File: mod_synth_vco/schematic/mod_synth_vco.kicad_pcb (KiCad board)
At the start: 2 copper layers, 38.1 x 109.2 mm, 29 parts, among them J1 Saw, J2 Triangle, J3 Conn_02x08_Odd_Even, J4 Freq CV, J5 PWM CV, J6 Square, U1 TL072, U2 AS3340, U3 TL072

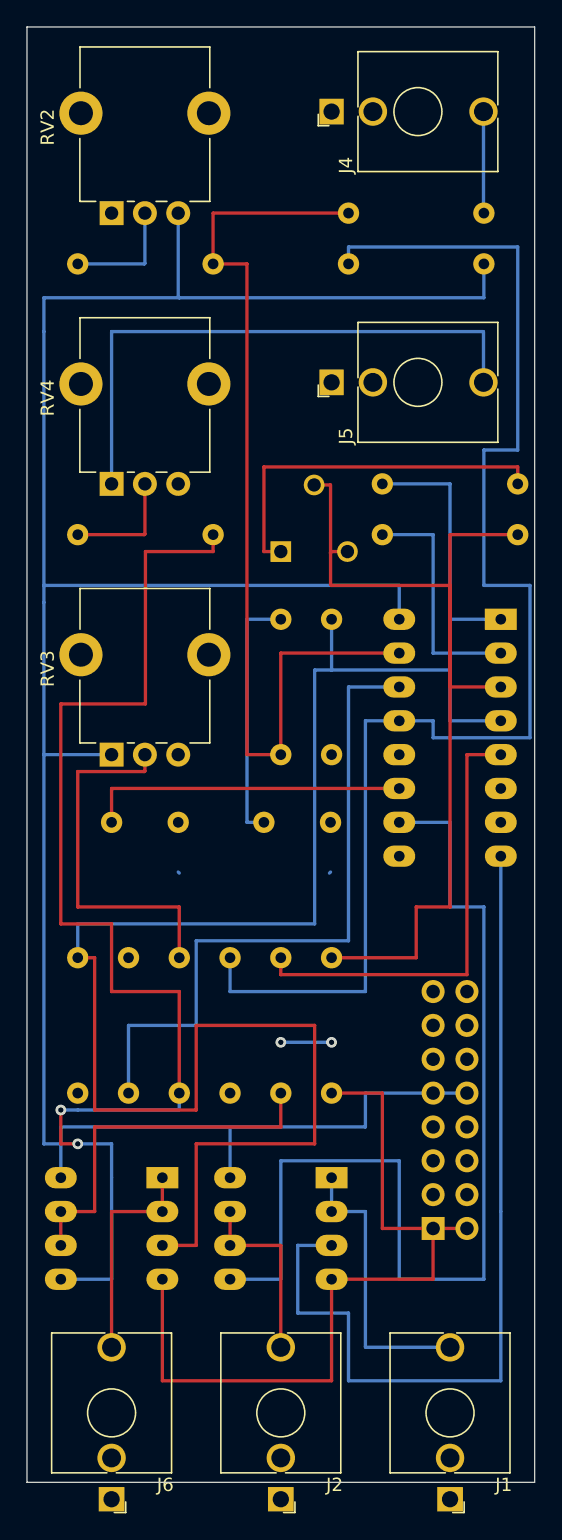
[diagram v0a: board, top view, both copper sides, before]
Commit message: Update PCB layouts
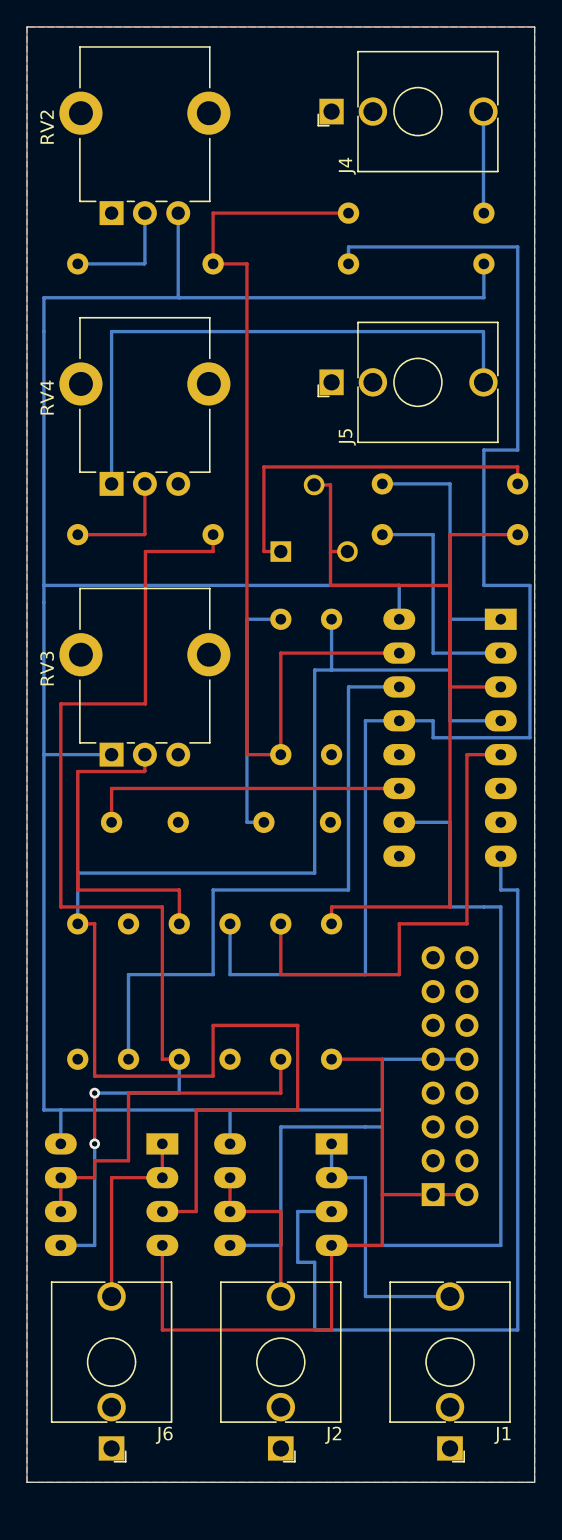
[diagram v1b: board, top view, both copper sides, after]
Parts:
- moved J1 3.81 mm to (69.8, 132.1)
- moved J2 3.81 mm to (57.1, 132.1)
- moved J6 3.81 mm to (44.5, 132.1)
- moved R10 2.54 mm to (41.9, 92.7)
- moved R14 2.54 mm to (57.1, 92.7)
- moved R2 2.54 mm to (61.0, 92.7)
- moved R5 2.54 mm to (53.3, 92.7)
- moved R6 2.54 mm to (45.7, 92.7)
- moved U1 2.54 mm to (61.0, 109.2)
- moved U3 2.54 mm to (48.3, 109.2)
- moved J3 2.54 mm to (68.6, 113.0)
- moved R12 2.54 mm to (49.5, 102.9)
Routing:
- net Net-(R10-Pad1): track 124.5 -> 114.3 mm
- net Net-(R12-Pad1): track 92.7 -> 82.6 mm
- net -12V: track 59.7 -> 53.3 mm
- net GND: track 4.15 -> 0.11 mm, vias 2 -> 0
- net +12V: track 181.6 -> 177.8 mm
- net Net-(R14-Pad1): track 34.3 -> 36.8 mm
- net Net-(R12-Pad2): track 27.9 -> 25.3 mm
- net Net-(U1-Pad3): track 67.3 -> 64.8 mm
- net Net-(R6-Pad2): track 50.8 -> 48.3 mm
- net Net-(R2-Pad1): track 76.1 -> 73.6 mm
- net Net-(J2-PadT): track 14.0 -> 12.7 mm
- net Net-(J6-PadT): track 16.5 -> 15.3 mm
- net Net-(J1-PadT): track 21.6 -> 20.3 mm
- added copper zone on B.Cu, net GND
- added copper zone on F.Cu, net GND
